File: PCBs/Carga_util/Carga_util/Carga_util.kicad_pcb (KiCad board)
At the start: 2 copper layers, 19 parts

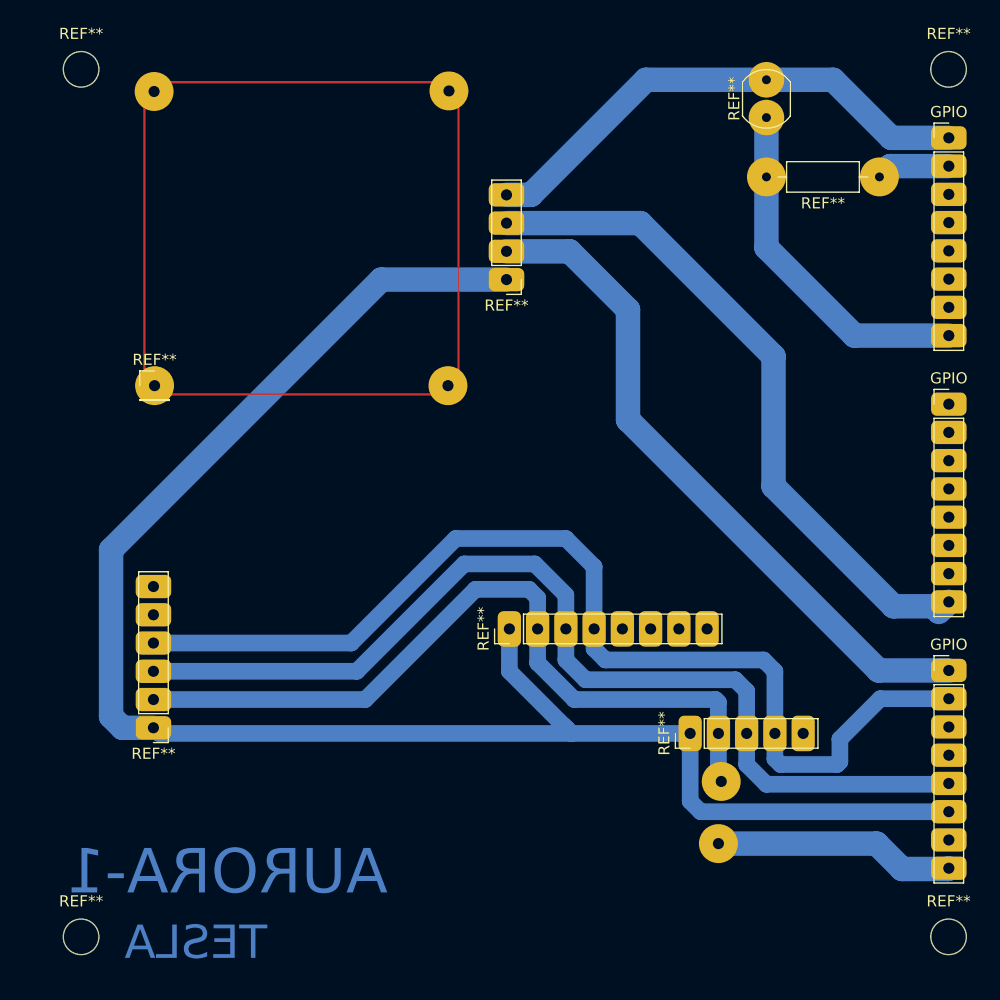
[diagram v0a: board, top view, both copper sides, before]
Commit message: Update Carga_util.kicad_pcb
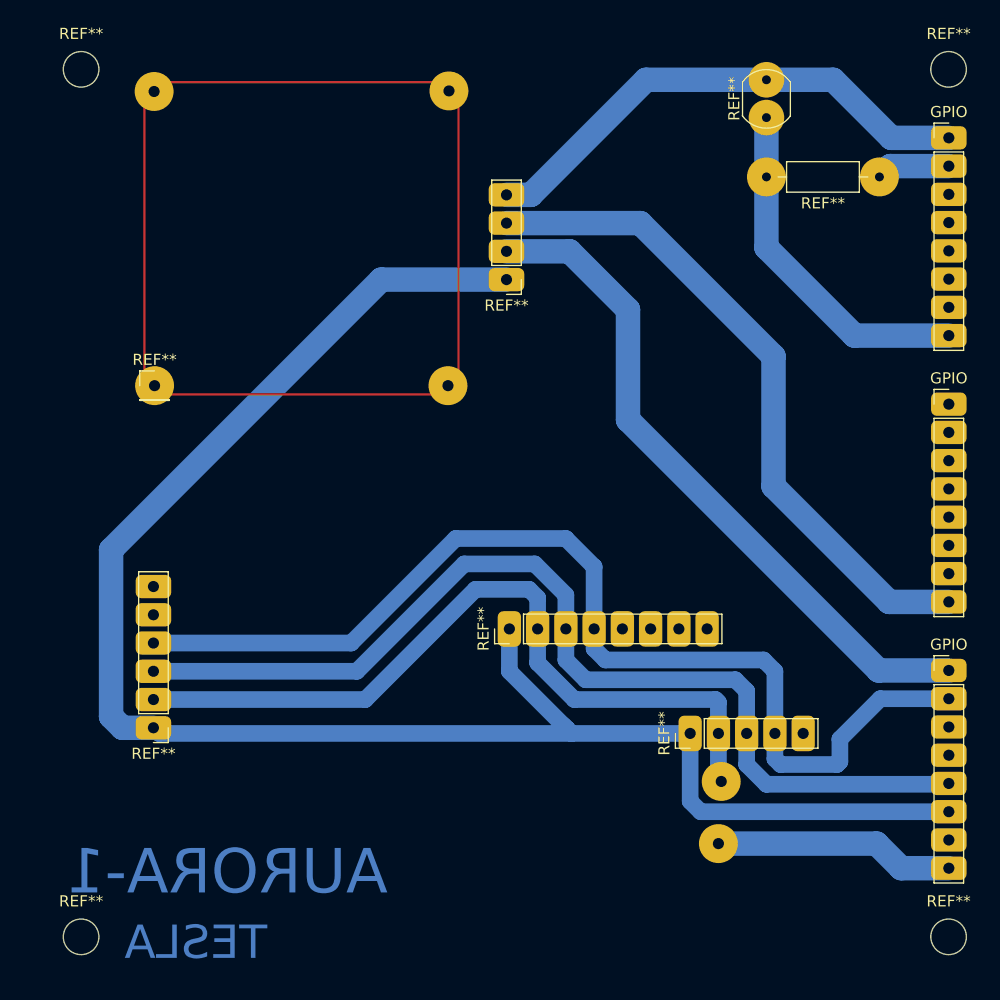
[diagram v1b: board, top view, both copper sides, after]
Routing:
- net (no net): track 642.0 -> 640.3 mm
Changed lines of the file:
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@@
   (segment (start 159.512 56.544) (end 148.678 56.544) (width 2.2) (layer "B.Cu") (net 0))
   (segment (start 147.066 87.122) (end 169.599 109.655) (width 2.2) (layer "B.Cu") (net 0))
-  (segment (start 160.147 93.091) (end 170.942 103.886) (width 2.2) (layer "B.Cu") (net 0))
-  (segment (start 170.942 103.886) (end 175.514 103.886) (width 2.2) (layer "B.Cu") (net 0))
   (segment (start 141.224 114.554) (end 141.605 114.935) (width 1.5) (layer "B.Cu") (net 0))
-  (segment (start 148.17 69.43) (end 160.147 81.407) (width 2.2) (layer "B.Cu") (net 0))
   (segment (start 136.14 74.51) (end 124.88 74.51) (width 2.2) (layer "B.Cu") (net 0))
   (segment (start 160.782 118.11) (end 165.862 118.11) (width 1.5) (layer "B.Cu") (net 0))
@@
   (segment (start 138.938 103.124) (end 138.938 105.918) (width 1.5) (layer "B.Cu") (net 0))
   (segment (start 154.94 112.268) (end 155.194 112.522) (width 1.5) (layer "B.Cu") (net 0))
+  (segment (start 160.147 93.091) (end 160.147 81.407) (width 2.2) (layer "B.Cu") (net 0))
+  (segment (start 175.91 103.49) (end 170.546 103.49) (width 2.2) (layer "B.Cu") (net 0))
   (segment (start 170.731 61.765) (end 165.51 56.544) (width 2.2) (layer "B.Cu") (net 0))
   (segment (start 156.718 110.49) (end 157.734 111.506) (width 1.5) (layer "B.Cu") (net 0))
@@
   (segment (start 143.256 110.49) (end 156.718 110.49) (width 1.5) (layer "B.Cu") (net 0))
   (segment (start 170.645 64.305) (end 169.672 65.278) (width 2.2) (layer "B.Cu") (net 0))
+  (segment (start 170.546 103.49) (end 160.147 93.091) (width 2.2) (layer "B.Cu") (net 0))
   (segment (start 147.066 77.216) (end 147.066 87.122) (width 2.2) (layer "B.Cu") (net 0))
   (segment (start 153.597 122.355) (end 175.91 122.355) (width 1.5) (layer "B.Cu") (net 0))
-  (segment (start 169.418 125.222) (end 171.704 127.508) (width 2.2) (layer "B.Cu") (net 0))
+  (segment (start 160.147 81.407) (end 148.17 69.43) (width 2.2) (layer "B.Cu") (net 0))
   (segment (start 141.478 97.79) (end 144.018 100.33) (width 1.5) (layer "B.Cu") (net 0))
-  (segment (start 175.837 127.508) (end 175.91 127.435) (width 2.2) (layer "B.Cu") (net 0))
   (segment (start 175.91 112.195) (end 169.745 112.195) (width 1.5) (layer "B.Cu") (net 0))
-  (segment (start 175.91 103.49) (end 175.006 104.394) (width 2.2) (layer "B.Cu") (net 0))
   (segment (start 141.478 102.87) (end 141.478 105.918) (width 1.5) (layer "B.Cu") (net 0))
   (segment (start 155.194 119.38) (end 155.448 119.634) (width 1.5) (layer "B.Cu") (net 0))
@@
   (segment (start 159.512 59.944) (end 159.512 65.278) (width 2.2) (layer "B.Cu") (net 0))
   (segment (start 159.512 65.278) (end 159.512 71.628) (width 2.2) (layer "B.Cu") (net 0))
-  (segment (start 136.14 69.43) (end 148.17 69.43) (width 2.2) (layer "B.Cu") (net 0))
   (segment (start 160.274 117.602) (end 160.782 118.11) (width 1.5) (layer "B.Cu") (net 0))
   (segment (start 152.654 121.412) (end 153.597 122.355) (width 1.5) (layer "B.Cu") (net 0))
@@
   (segment (start 157.734 115.316) (end 157.734 118.11) (width 1.5) (layer "B.Cu") (net 0))
   (segment (start 175.837 119.888) (end 175.91 119.815) (width 1.5) (layer "B.Cu") (net 0))
-  (segment (start 160.147 81.407) (end 160.147 93.091) (width 2.2) (layer "B.Cu") (net 0))
   (segment (start 145.034 108.712) (end 159.258 108.712) (width 1.5) (layer "B.Cu") (net 0))
   (segment (start 104.394 109.728) (end 122.682 109.728) (width 1.5) (layer "B.Cu") (net 0))
+  (segment (start 171.631 127.435) (end 169.418 125.222) (width 2.2) (layer "B.Cu") (net 0))
   (segment (start 141.986 115.316) (end 152.654 115.316) (width 1.5) (layer "B.Cu") (net 0))
   (segment (start 166.116 115.824) (end 166.116 117.856) (width 1.5) (layer "B.Cu") (net 0))
@@
   (segment (start 141.605 114.935) (end 141.986 115.316) (width 1.5) (layer "B.Cu") (net 0))
   (segment (start 138.938 105.918) (end 138.938 108.966) (width 1.5) (layer "B.Cu") (net 0))
+  (segment (start 175.91 127.435) (end 171.631 127.435) (width 2.2) (layer "B.Cu") (net 0))
   (segment (start 136.14 71.97) (end 141.82 71.97) (width 2.2) (layer "B.Cu") (net 0))
   (segment (start 144.018 105.918) (end 144.018 107.696) (width 1.5) (layer "B.Cu") (net 0))
   (segment (start 104.902 115.316) (end 104.394 114.808) (width 1.5) (layer "B.Cu") (net 0))
-  (segment (start 175.514 103.886) (end 175.91 103.49) (width 2.2) (layer "B.Cu") (net 0))
   (segment (start 165.51 56.544) (end 159.512 56.544) (width 2.2) (layer "B.Cu") (net 0))
   (segment (start 122.682 109.728) (end 132.334 100.076) (width 1.5) (layer "B.Cu") (net 0))
@@
   (segment (start 144.018 107.696) (end 145.034 108.712) (width 1.5) (layer "B.Cu") (net 0))
   (segment (start 159.512 119.888) (end 175.837 119.888) (width 1.5) (layer "B.Cu") (net 0))
-  (segment (start 171.704 127.508) (end 175.837 127.508) (width 2.2) (layer "B.Cu") (net 0))
   (segment (start 175.91 64.305) (end 170.645 64.305) (width 2.2) (layer "B.Cu") (net 0))
   (segment (start 123.444 112.268) (end 133.35 102.362) (width 1.5) (layer "B.Cu") (net 0))
@@
   (segment (start 136.398 105.918) (end 136.398 109.728) (width 1.5) (layer "B.Cu") (net 0))
   (segment (start 155.194 112.522) (end 155.194 115.316) (width 1.5) (layer "B.Cu") (net 0))
+  (segment (start 148.17 69.43) (end 136.14 69.43) (width 2.2) (layer "B.Cu") (net 0))
 )
